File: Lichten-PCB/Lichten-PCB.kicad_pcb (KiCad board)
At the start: 2 copper layers, 54.2 x 62.2 mm, 56 parts, among them J1 Conn_01x04_Socket

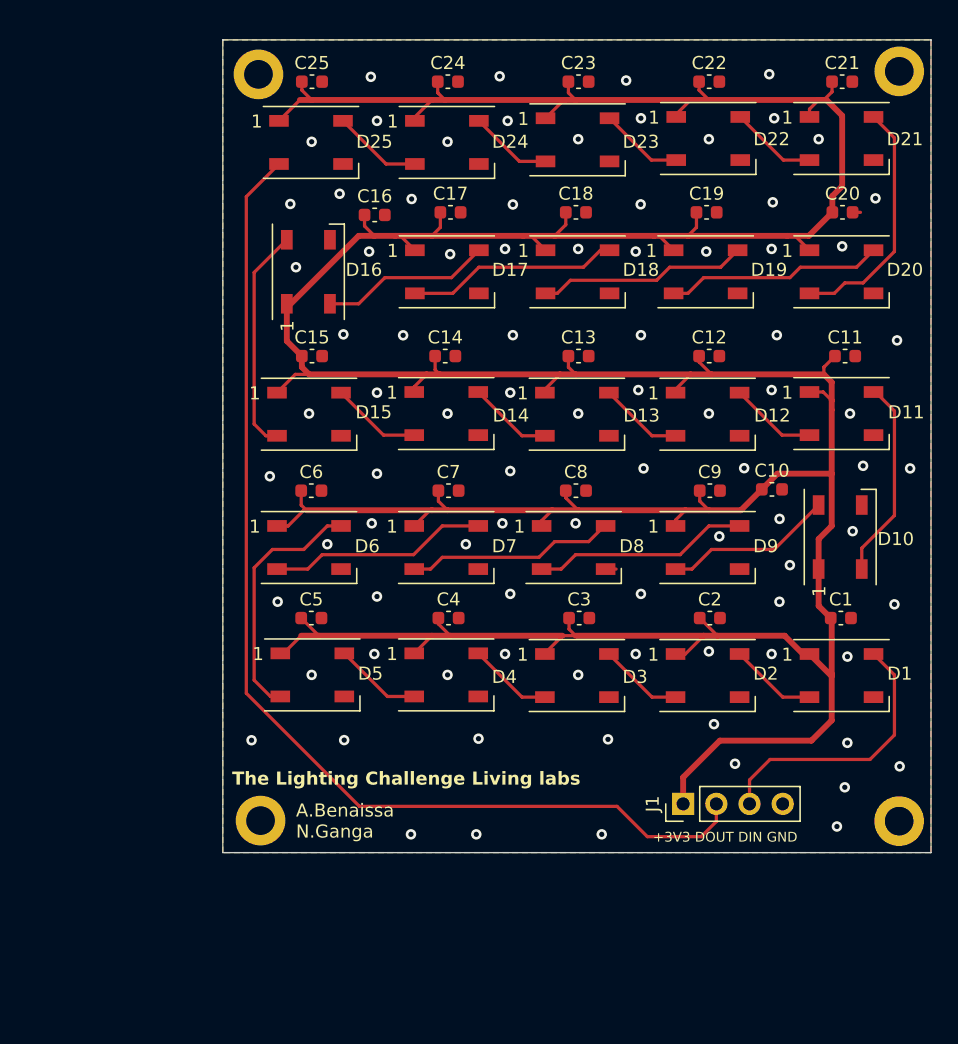
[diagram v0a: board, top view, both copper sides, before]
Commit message: PCB vergroot
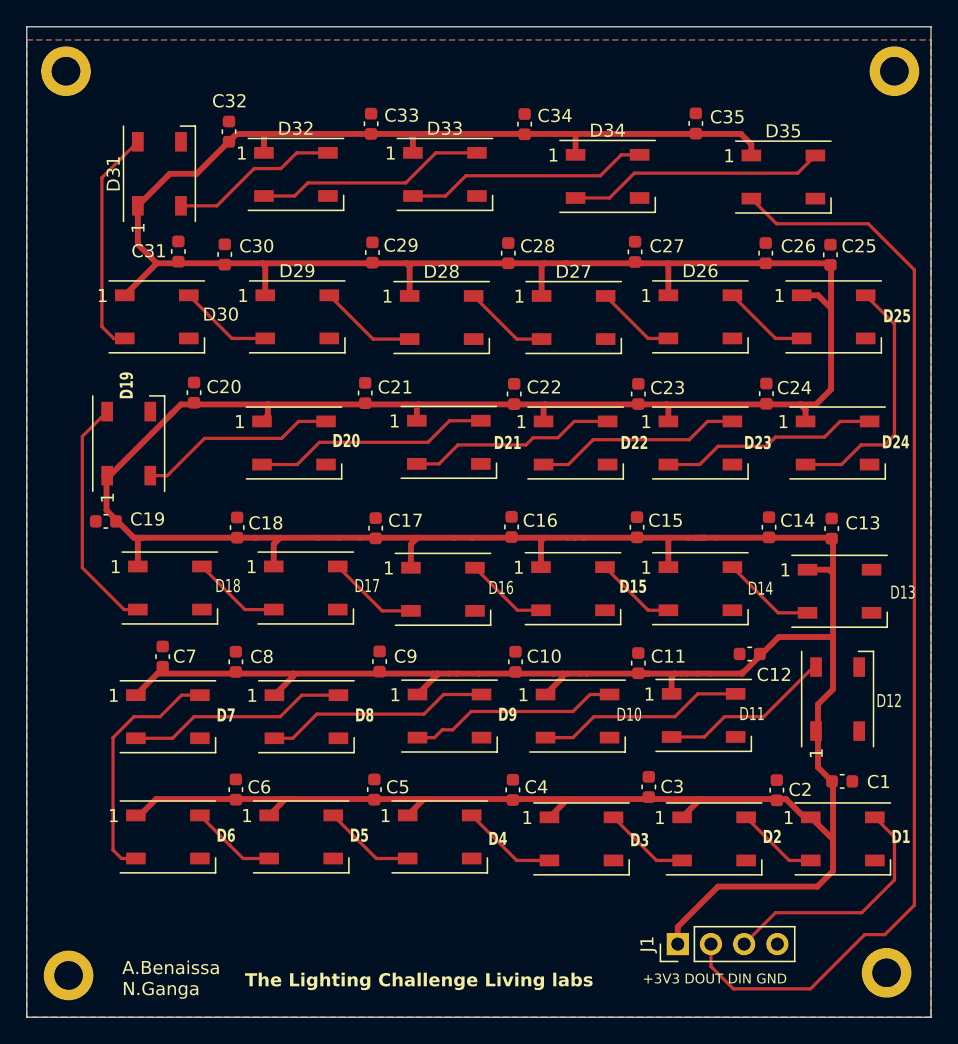
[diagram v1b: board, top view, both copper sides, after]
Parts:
- added C26: 0.1u, Capacitor_SMD:C_0603_1608Metric, F.Cu at (159.8, 86.3)
- added C27: 0.1u, Capacitor_SMD:C_0603_1608Metric, F.Cu at (149.8, 86.2)
- added C28: 0.1u, Capacitor_SMD:C_0603_1608Metric, F.Cu at (140.1, 86.3)
- added C29: 0.1u, Capacitor_SMD:C_0603_1608Metric, F.Cu at (129.7, 86.3)
- added C30: 0.1u, Capacitor_SMD:C_0603_1608Metric, F.Cu at (118.3, 86.4)
- added C31: 0.1u, Capacitor_SMD:C_0603_1608Metric, F.Cu at (114.8, 86.2)
- added C32: 0.1u, Capacitor_SMD:C_0603_1608Metric, F.Cu at (118.7, 77.0)
- added C33: 0.1u, Capacitor_SMD:C_0603_1608Metric, F.Cu at (129.6, 76.4)
- added C34: 0.1u, Capacitor_SMD:C_0603_1608Metric, F.Cu at (141.3, 76.5)
- added C35: 0.1u, Capacitor_SMD:C_0603_1608Metric, F.Cu at (154.4, 76.4)
- added D26: WS2812B, LED_SMD:LED_WS2812B_PLCC4_5.0x5.0mm_P3.2mm, F.Cu at (154.8, 91.2)
- added D27: WS2812B, LED_SMD:LED_WS2812B_PLCC4_5.0x5.0mm_P3.2mm, F.Cu at (145.1, 91.2)
- added D28: WS2812B, LED_SMD:LED_WS2812B_PLCC4_5.0x5.0mm_P3.2mm, F.Cu at (134.9, 91.2)
- added D29: WS2812B, LED_SMD:LED_WS2812B_PLCC4_5.0x5.0mm_P3.2mm, F.Cu at (123.9, 91.2)
- added D30: WS2812B, LED_SMD:LED_WS2812B_PLCC4_5.0x5.0mm_P3.2mm, F.Cu at (113.2, 91.2)
- added D31: WS2812B, LED_SMD:LED_WS2812B_PLCC4_5.0x5.0mm_P3.2mm, F.Cu at (113.3, 80.2)
- added D32: WS2812B, LED_SMD:LED_WS2812B_PLCC4_5.0x5.0mm_P3.2mm, F.Cu at (123.8, 80.3)
- added D33: WS2812B, LED_SMD:LED_WS2812B_PLCC4_5.0x5.0mm_P3.2mm, F.Cu at (135.2, 80.3)
- added D34: WS2812B, LED_SMD:LED_WS2812B_PLCC4_5.0x5.0mm_P3.2mm, F.Cu at (147.7, 80.5)
- added D35: WS2812B, LED_SMD:LED_WS2812B_PLCC4_5.0x5.0mm_P3.2mm, F.Cu at (161.1, 80.5)
- moved C19 51.7 mm to (109.2, 106.8), turned to 180 degrees
- moved C20 51.5 mm to (116.0, 97.0), turned to 90 degrees
- moved D19 46.1 mm to (111.0, 100.9), turned to 90 degrees
- moved D20 43.9 mm to (123.7, 100.8)
- moved C21 43.6 mm to (129.1, 97.0), turned to 90 degrees
- moved D25 42.2 mm to (164.9, 91.2)
- moved C25 41.8 mm to (164.7, 86.5), turned to 90 degrees
- moved D18 39.5 mm to (114.2, 112.0)
- moved D21 38.0 mm to (135.5, 100.8)
- moved D24 37.7 mm to (165.2, 100.8)
- moved C18 35.4 mm to (119.3, 107.3), turned to 90 degrees
- moved C24 34.1 mm to (159.8, 97.1), turned to 90 degrees
- moved C8 29.1 mm to (119.2, 117.6), turned to 90 degrees
- moved C9 28.5 mm to (130.2, 117.6), turned to 90 degrees
- moved C11 28.3 mm to (150.0, 117.7), turned to 90 degrees
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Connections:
- net DTUS renamed DTUS1
- D25 pad 2: DOUT -> DTUS2
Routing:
- net +3V3: track 348.3 -> 445.0 mm
- net /LED's/Data-33: track 0.00 -> 19.7 mm
- net /LED's/Data-32: track 0.00 -> 18.7 mm
- net /LED's/Data-31: track 0.00 -> 17.7 mm
- net /LED's/Data-29: track 0.00 -> 17.4 mm
- net /LED's/Data-30: track 0.00 -> 12.9 mm
- net /LED's/Data-24: track 6.87 -> 19.3 mm
- net /LED's/Data-5: track 19.1 -> 6.67 mm
- net /LED's/Data-15: track 17.3 -> 6.40 mm
- net /LED's/Data-23: track 6.38 -> 16.8 mm
- net /LED's/Data-17: track 16.3 -> 6.87 mm
- net /LED's/Data-22: track 6.43 -> 15.8 mm
- net /LED's/Data-21: track 6.67 -> 15.9 mm
- net /LED's/Data-27: track 0.00 -> 7.54 mm
- net /LED's/Data-28: track 0.00 -> 7.22 mm
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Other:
- board size 54.2 x 62.2 mm -> 69.2 x 75.8 mm
- board text added: "D6"
